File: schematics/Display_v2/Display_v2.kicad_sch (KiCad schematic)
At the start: 9 parts, among them J1 Conn_01x02_Pin, J2 Conn_01x04_Pin, M1 Stepper_Motor_bipolar, SW2 SW_SPST

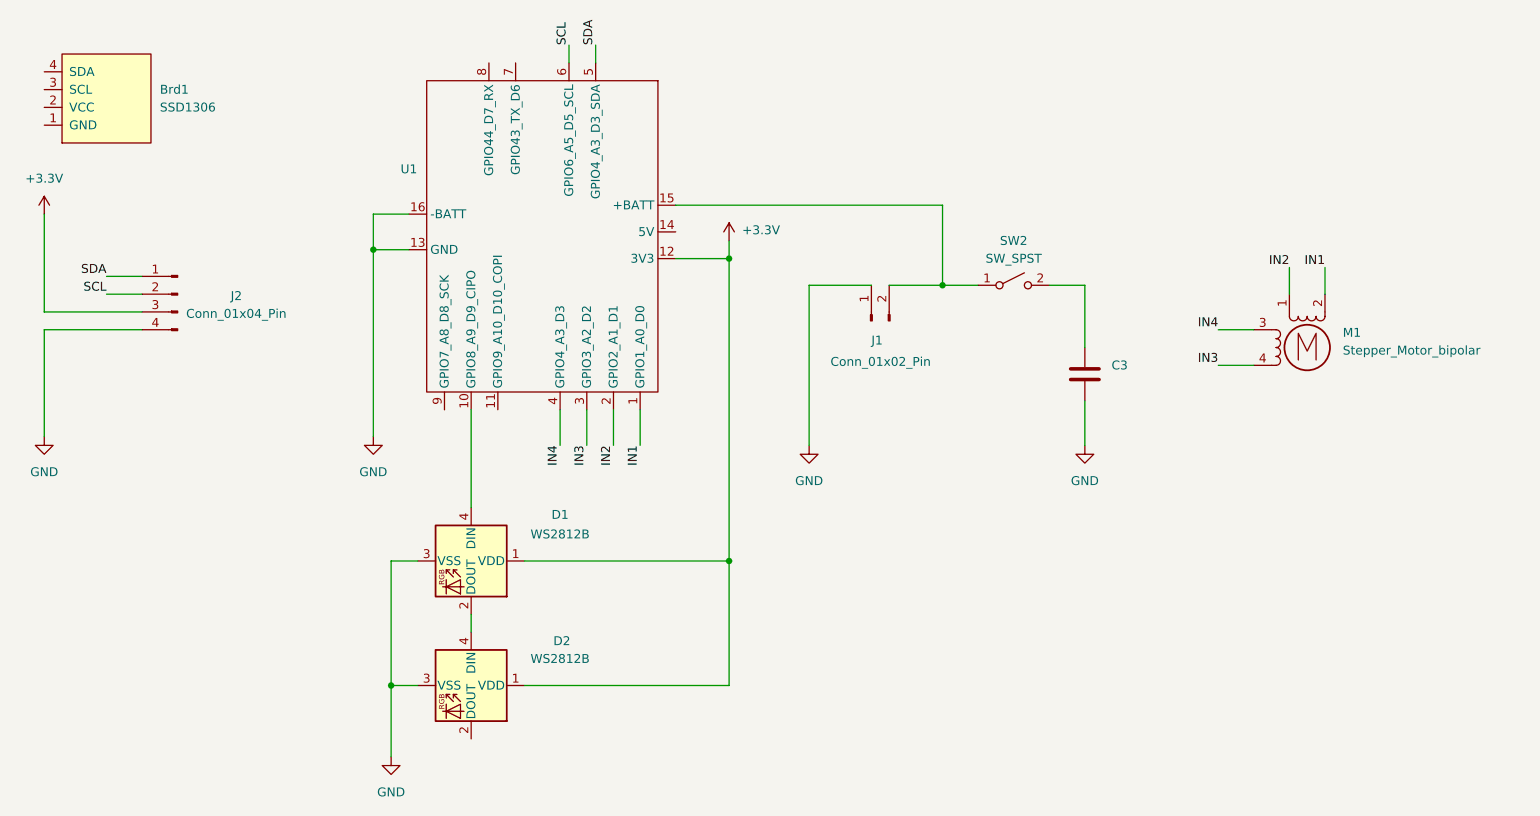
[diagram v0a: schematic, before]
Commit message: Update code
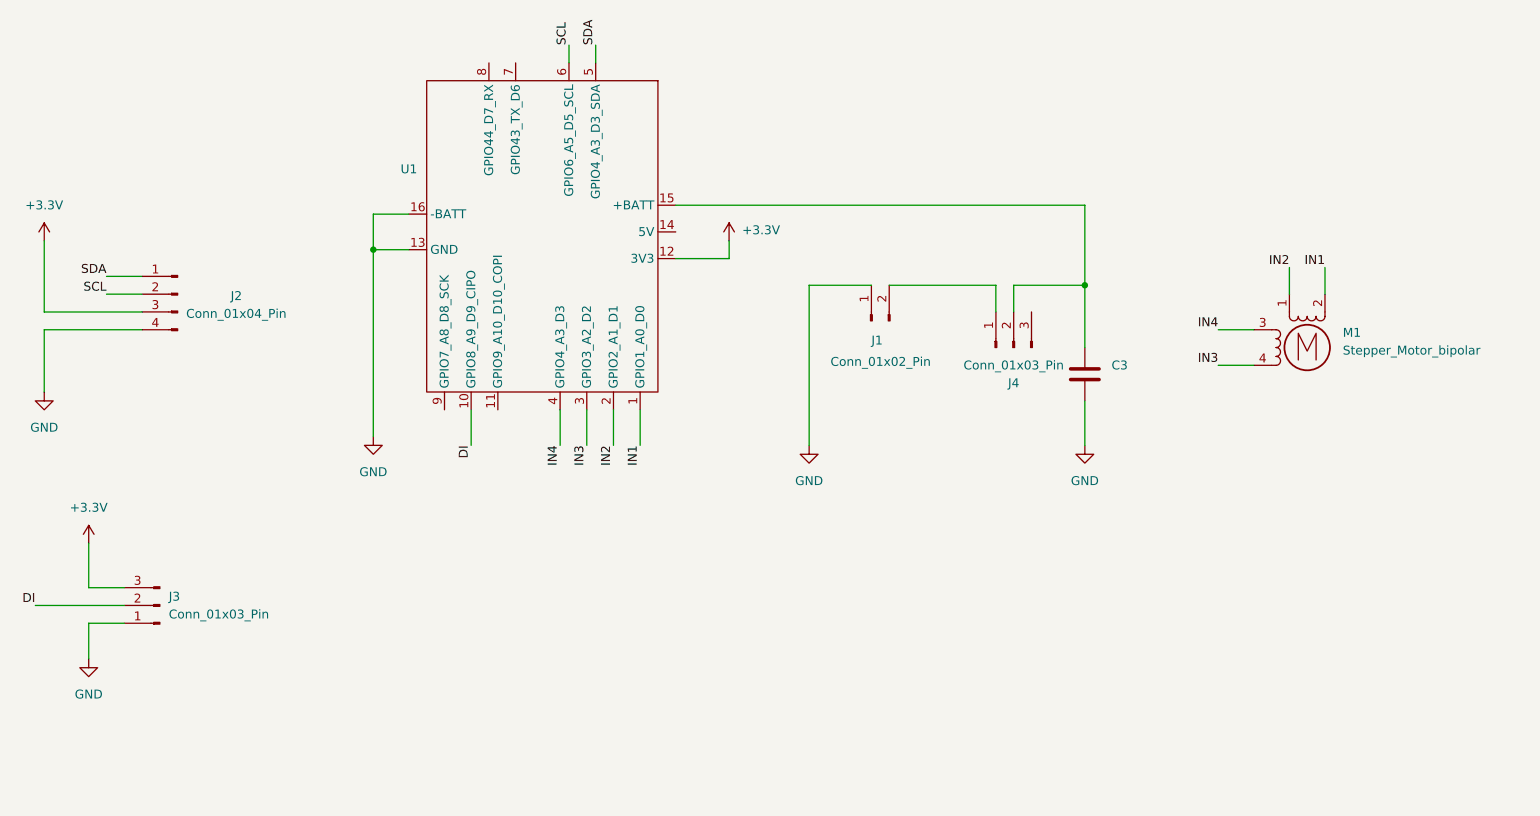
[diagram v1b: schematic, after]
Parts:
- removed Brd1: SSD1306, Display:Adafruit_SSD1306_No_Mounting_Holes, symbol sensorcircuits:SSD1306
- removed D1, D2: WS2812B, LED_SMD:LED_WS2812B_PLCC4_5.0x5.0mm_P3.2mm, symbol LED:WS2812B
- removed SW2: SW_SPST, Button_Switch_SMD:SW_DIP_SPSTx01_Slide_6.7x4.1mm_W6.73mm_P2.54mm_LowProfile_JPin, symbol Switch:SW_SPST
- added J3, J4: Conn_01x03_Pin, Connector_PinSocket_2.54mm:PinSocket_1x03_P2.54mm_Vertical, symbol Connector:Conn_01x03_Pin
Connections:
- net +3.3V: now also J3.3 (Pin_3)
- net GND: now also J3.1 (Pin_1)
- net DI: now reaches U1.10 (GPIO8_A9_D9_CIPO)
- net DI: now also J3.2 (Pin_2)
- net at U1.15 (+BATT): now also C3.1, J4.2 (Pin_2); no longer J1.2 (Pin_2)
- new net: J1.2 (Pin_2), J4.1 (Pin_1)
